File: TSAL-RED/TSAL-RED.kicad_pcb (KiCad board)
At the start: 2 copper layers, 81.9 x 61.6 mm, 43 parts, among them J1 Conn_01x02, J2 Conn_01x02, J5 Conn_02x01, J6 Conn_02x03_Counter_Clockwise, K1 G5V-2, Q1 2N7002, Q2 AO3401A, U1 LM358, U2 4N35, U3 NE555D

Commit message: Corrected voltage threshold to 50.4V
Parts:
- R15: value 270 -> 150
- R2: value 10K -> 12K
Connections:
- net /Vin renamed /V_Cap
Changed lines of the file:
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@@
 	(net 9 "Net-(Q1-D)")
 	(net 10 "Net-(Q2-G)")
-	(net 11 "/Vin")
+	(net 11 "/V_Cap")
 	(net 12 "Net-(R3-Pad1)")
 	(net 13 "Net-(R3-Pad2)")
@@
 			)
 		)
-		(property "Datasheet" ""
+		(property "Datasheet" "~"
 			(at 0 0 270)
 			(unlocked yes)
@@
 			)
 		)
-		(property "Datasheet" ""
+		(property "Datasheet" "~"
 			(at 0 0 270)
 			(unlocked yes)
@@
 			)
 		)
-		(property "Datasheet" ""
+		(property "Datasheet" "~"
 			(at 0 0 270)
 			(unlocked yes)
@@
 			(layers "F.Cu" "F.Mask" "F.Paste")
 			(roundrect_rratio 0.192308)
-			(net 11 "/Vin")
+			(net 11 "/V_Cap")
 			(pintype "passive")
 		)
@@
 			)
 		)
-		(property "Datasheet" ""
+		(property "Datasheet" "~"
 			(at 0 0 90)
 			(unlocked yes)
@@
 			)
 		)
-		(property "Datasheet" ""
+		(property "Datasheet" "~"
 			(at 0 0 270)
 			(unlocked yes)
@@
 			)
 		)
-		(property "Datasheet" ""
+		(property "Datasheet" "~"
 			(at 0 0 270)
 			(unlocked yes)
@@
 			)
 		)
-		(property "Datasheet" ""
+		(property "Datasheet" "~"
 			(at 0 0 0)
 			(unlocked yes)
@@
 			)
 		)
-		(property "Datasheet" ""
+		(property "Datasheet" "~"
 			(at 0 0 90)
 			(unlocked yes)
@@
 			)
 		)
-		(property "Datasheet" ""
+		(property "Datasheet" "~"
 			(at 0 0 0)
 			(unlocked yes)
@@
 			)
 		)
-		(property "Datasheet" ""
+		(property "Datasheet" "~"
 			(at 0 0 180)
 			(unlocked yes)
@@
 			)
 		)
-		(property "Datasheet" ""
+		(property "Datasheet" "~"
 			(at 0 0 90)
 			(unlocked yes)
@@
 			)
 		)
-		(property "Datasheet" ""
+		(property "Datasheet" "~"
 			(at 0 0 180)
 			(unlocked yes)
@@
 			)
 		)
-		(property "Value" "270"
+		(property "Value" "150"
 			(at 0 1.83 90)
 			(layer "F.Fab")
@@
 			)
 		)
-		(property "Datasheet" ""
+		(property "Datasheet" "~"
 			(at 0 0 90)
 			(layer "F.Fab")
@@
 			)
 		)
-		(property "Datasheet" ""
+		(property "Datasheet" "~"
 			(at 0 0 90)
 			(unlocked yes)
@@
 			)
 		)
-		(property "Datasheet" ""
+		(property "Datasheet" "~"
 			(at 0 0 90)
 			(unlocked yes)
@@
 			)
 		)
-		(property "Datasheet" ""
+		(property "Datasheet" "~"
 			(at 0 0 180)
 			(unlocked yes)
@@
 			)
 		)
-		(property "Datasheet" ""
+		(property "Datasheet" "~"
 			(at 0 0 180)
 			(unlocked yes)
@@
 			)
 		)
-		(property "Datasheet" ""
+		(property "Datasheet" "~"
 			(at 0 0 90)
 			(unlocked yes)
@@
 			)
 		)
-		(property "Datasheet" ""
+		(property "Datasheet" "~"
 			(at 0 0 90)
 			(unlocked yes)
@@
 			)
 		)
-		(property "Datasheet" ""
+		(property "Datasheet" "~"
 			(at 0 0 0)
 			(unlocked yes)
@@
 			)
 		)
-		(property "Datasheet" ""
+		(property "Datasheet" "~"
 			(at 0 0 180)
 			(unlocked yes)
@@
 			)
 		)
-		(property "Datasheet" ""
+		(property "Datasheet" "~"
 			(at 0 0 180)
 			(unlocked yes)
@@
 			)
 		)
-		(property "Datasheet" ""
+		(property "Datasheet" "~"
 			(at 0 0 270)
 			(unlocked yes)
@@
 			)
 		)
-		(property "Datasheet" ""
+		(property "Datasheet" "~"
 			(at 0 0 180)
 			(unlocked yes)
@@
 			)
 		)
-		(property "Datasheet" ""
+		(property "Datasheet" "~"
 			(at 0 0 90)
 			(unlocked yes)
@@
 			)
 		)
-		(property "Datasheet" ""
+		(property "Datasheet" "~"
 			(at 0 0 180)
 			(unlocked yes)
@@
 			)
 		)
-		(property "Datasheet" ""
+		(property "Datasheet" "~"
 			(at 0 0 90)
 			(unlocked yes)
@@
 			)
 		)
-		(property "Datasheet" ""
+		(property "Datasheet" "~"
 			(at 0 0 0)
 			(unlocked yes)
@@
 			)
 		)
-		(property "Datasheet" ""
+		(property "Datasheet" "~"
 			(at 0 0 270)
 			(unlocked yes)
@@
 			)
 		)
-		(property "Datasheet" ""
+		(property "Datasheet" "~"
 			(at 0 0 180)
 			(unlocked yes)
@@
 			)
 		)
-		(property "Datasheet" ""
+		(property "Datasheet" "~"
 			(at 0 0 0)
 			(unlocked yes)
@@
 			(layers "F.Cu" "F.Mask" "F.Paste")
 			(roundrect_rratio 0.25)
-			(net 11 "/Vin")
+			(net 11 "/V_Cap")
 			(pinfunction "-")
 			(pintype "input")
@@
 			)
 		)
-		(property "Value" "10K"
+		(property "Value" "12K"
 			(at 0 1.82 90)
 			(layer "F.Fab")
@@
 			)
 		)
-		(property "Datasheet" ""
+		(property "Datasheet" "~"
 			(at 0 0 270)
 			(unlocked yes)
@@
 			(layers "F.Cu" "F.Mask" "F.Paste")
 			(roundrect_rratio 0.192308)
-			(net 11 "/Vin")
+			(net 11 "/V_Cap")
 			(pintype "passive")
 		)

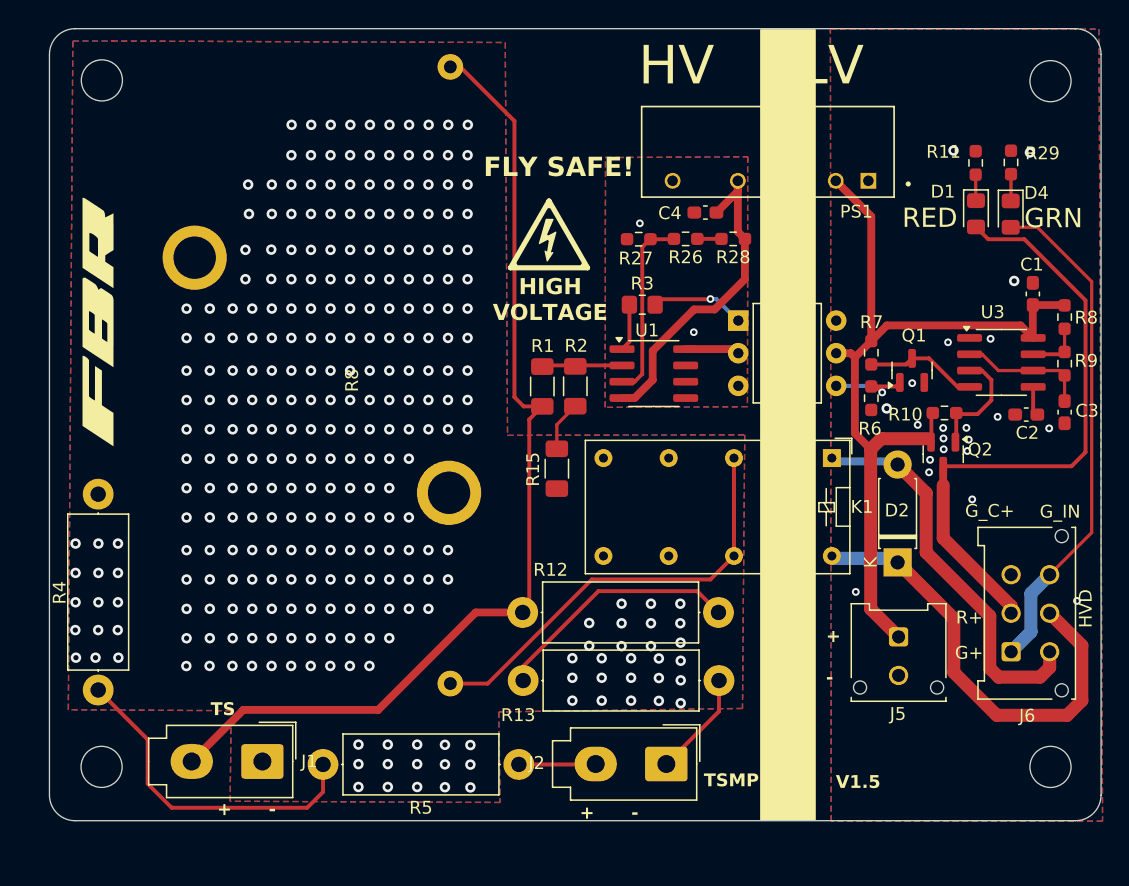
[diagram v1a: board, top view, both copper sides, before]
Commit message: Save corrupted files and new modifications
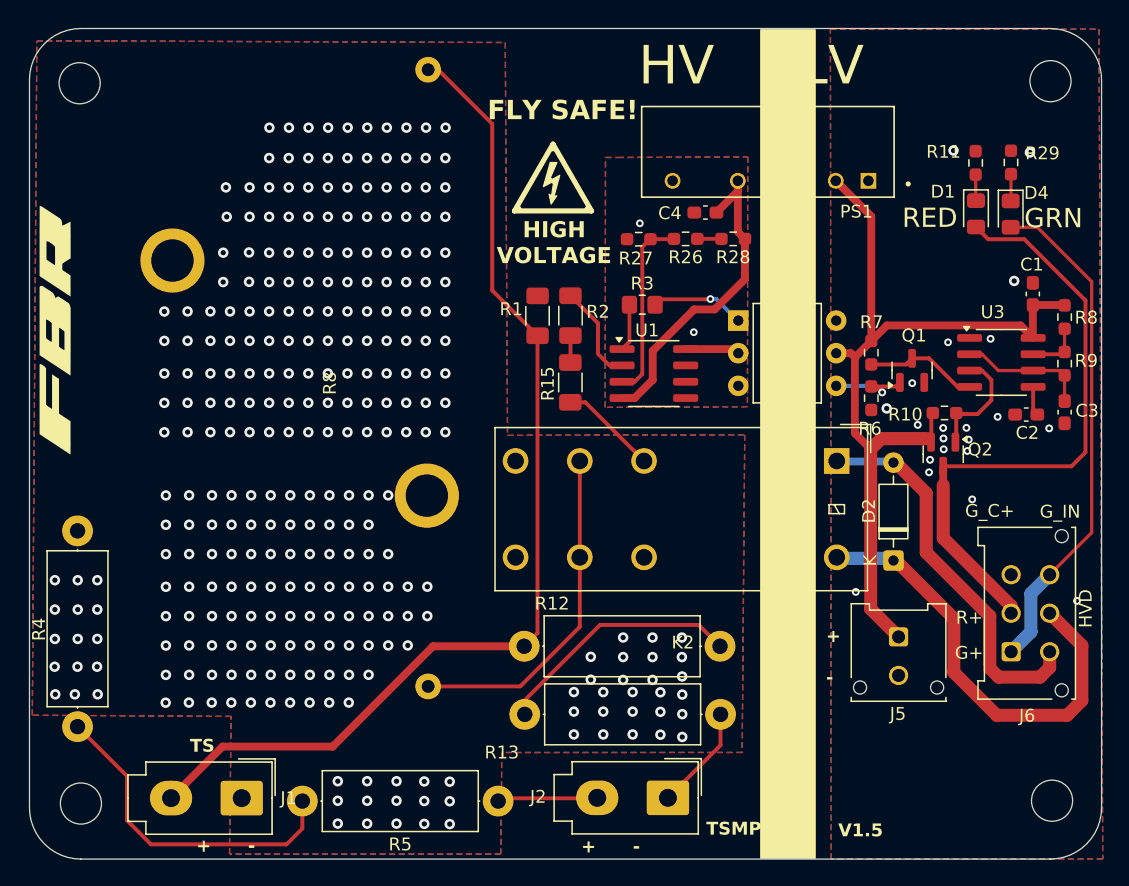
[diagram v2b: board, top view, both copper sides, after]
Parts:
- removed K1: G5V-2, Relay_THT:Relay_DPDT_Omron_G5V-2
- added K2: G2RL-1-E, Relay_THT:Relay_DPDT_Omron_G2RL-2, F.Cu at (112.5, 93.7)
- D2: value 1n4937 -> 1N4148; footprint Diode_THT:D_DO-41_SOD81_P7.62mm_Horizontal -> Diode_THT:D_DO-35_SOD27_P7.62mm_Horizontal
- moved R15 6.80 mm to (91.8, 87.6)
- moved R1 5.51 mm to (89.2, 82.4)
- moved R2 5.51 mm to (91.8, 82.4)
- moved REF** 4.44 mm to (90.5, 71.7)
- moved G*** 3.40 mm to (51.6, 83.7)
- moved H2 3.28 mm to (53.7, 120.4)
- moved J1 3.28 mm to (66.2, 120.0)
- moved R4 3.28 mm to (53.4, 114.4)
- moved R5 3.28 mm to (86.2, 120.2)
- moved R13 2.63 mm to (103.5, 113.4)
- moved J2 2.63 mm to (99.4, 119.9)
- moved R12 2.63 mm to (103.5, 108.1)
- moved H3 2.63 mm to (129.3, 120.2)
- moved R14 1.74 mm to (70.7, 87.3)
- moved H1 1.74 mm to (53.6, 64.3)
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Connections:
- net AIR+_Sup renamed /AIR_Sup+
- net TSAC_GLV- renamed /TSAC_GLV-
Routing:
- net Net-(K2-Pad11): track 34.4 -> 26.7 mm
- net TS-: track 0.00 -> 7.53 mm
- net TS+: track 80.0 -> 83.6 mm
- net Net-(J2-Pin_2): track 7.74 -> 9.56 mm
- net /V_Cap: track 6.35 -> 7.89 mm
- net Net-(R12-Pad1): track 19.4 -> 18.3 mm
- net Net-(R15-Pad1): track 3.18 -> 2.10 mm
- net /AIR_Sup+: track 36.4 -> 35.8 mm
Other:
- board size 81.9 x 61.6 mm -> 83.5 x 64.7 mm
